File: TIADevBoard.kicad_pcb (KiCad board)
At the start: 2 copper layers, 24.1 x 33 mm, 23 parts, among them J1 Screw_Terminal_01x02, J2 Conn_Coaxial, J3 Conn_Coaxial, J4 Conn_02x03_Counter_Clockwise, J5 Conn_Coaxial, U2 OPA2387, U3 ADP3330-3.3

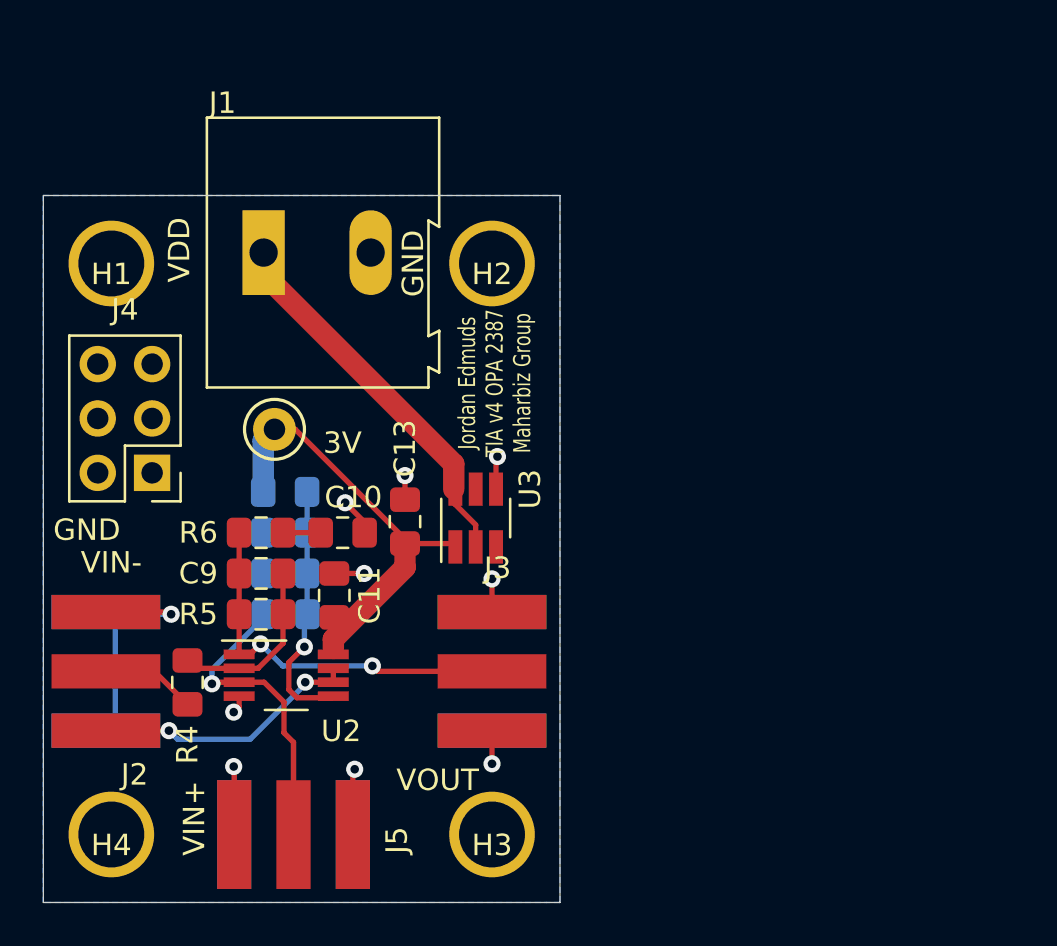
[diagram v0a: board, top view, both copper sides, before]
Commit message: added gerbers for version 5
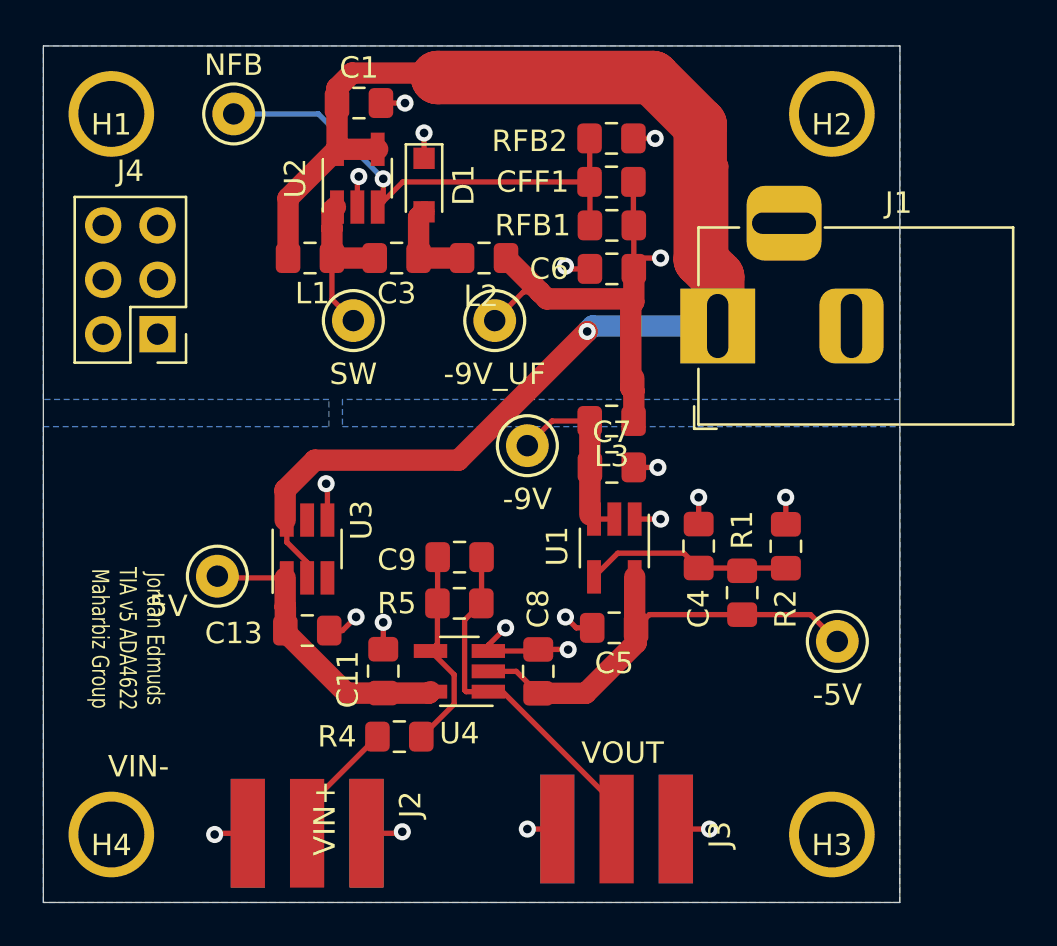
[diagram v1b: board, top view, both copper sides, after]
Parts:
- removed C10: 100pF, Capacitor_SMD:C_0805_2012Metric_Pad1.15x1.40mm_HandSolder
- removed J5: Conn_Coaxial, my_library_foot:CON-SMA-EDGE-S
- removed R3: 0R, Resistor_SMD:R_0805_2012Metric_Pad1.15x1.40mm_HandSolder
- removed R6: 1k, Resistor_SMD:R_0805_2012Metric_Pad1.15x1.40mm_HandSolder
- added C3: 1uF, Capacitor_SMD:C_0805_2012Metric_Pad1.15x1.40mm_HandSolder, F.Cu at (97.1, 82.3)
- added C4: 10nF, Capacitor_SMD:C_0805_2012Metric_Pad1.15x1.40mm_HandSolder, F.Cu at (111.3, 95.7)
- added C5: 10uF, Capacitor_SMD:C_0805_2012Metric_Pad1.15x1.40mm_HandSolder, F.Cu at (107.3, 99.6)
- added C6: 10uF, Capacitor_SMD:C_0805_2012Metric_Pad1.15x1.40mm_HandSolder, F.Cu at (107.2, 82.8)
- added C7: 10uF, Capacitor_SMD:C_0805_2012Metric_Pad1.15x1.40mm_HandSolder, F.Cu at (107.2, 92.1)
- added C8: 100nF, Capacitor_SMD:C_0805_2012Metric_Pad1.15x1.40mm_HandSolder, F.Cu at (103.8, 101.6)
- added CFF1: 100pF, Capacitor_SMD:C_0805_2012Metric_Pad1.15x1.40mm_HandSolder, F.Cu at (107.2, 78.7)
- added D1: D, Diode_SMD:D_SOD-323_HandSoldering, F.Cu at (98.4, 78.9)
- added L1: 22uH, Inductor_SMD:L_0805_2012Metric_Pad1.15x1.40mm_HandSolder, F.Cu at (93.1, 82.3)
- added L2: 22uH, Inductor_SMD:L_0805_2012Metric_Pad1.15x1.40mm_HandSolder, F.Cu at (101.2, 82.3)
- added L3: 22uH, Inductor_SMD:L_0805_2012Metric_Pad1.15x1.40mm_HandSolder, F.Cu at (107.2, 89.9)
- added RFB1: 30k, Resistor_SMD:R_0805_2012Metric_Pad1.15x1.40mm_HandSolder, F.Cu at (107.2, 80.8)
- added RFB2: 4.7k, Resistor_SMD:R_0805_2012Metric_Pad1.15x1.40mm_HandSolder, F.Cu at (107.2, 76.7)
- added TP2: -9V, my_library_foot:TestPoint_Keystone_5000-5004_Miniature, F.Cu at (103.3, 91.1)
- added TP3: -5V, my_library_foot:TestPoint_Keystone_5000-5004_Miniature, F.Cu at (117.7, 100.2)
- added TP4: -9V_UF, my_library_foot:TestPoint_Keystone_5000-5004_Miniature, F.Cu at (101.7, 85.2)
- added TP5: SW, my_library_foot:TestPoint_Keystone_5000-5004_Miniature, F.Cu at (95.1, 85.2)
- added TP6: NFB, my_library_foot:TestPoint_Keystone_5000-5004_Miniature, F.Cu at (89.5, 75.6)
- added U1: TPS723, Package_TO_SOT_SMD:SOT-23-5_HandSoldering, F.Cu at (107.3, 95.8)
- added U4: ADA4622, Package_TO_SOT_SMD:SOT-23-5_HandSoldering, F.Cu at (100.1, 101.6)
- C1: value C -> 10uF; moved to F.Cu
- C11: value 1uF -> 100nF
- J1: value Screw_Terminal_01x02 -> Jack-DC; footprint TerminalBlock:TerminalBlock_Altech_AK300-2_P5.00mm -> Connector_BarrelJack:BarrelJack_Horizontal
- R1: value 10k -> 32k; moved to F.Cu
- R2: value 10k -> 100k; moved to F.Cu
- TP1: value 3V -> 5V
- U2: value OPA2387 -> LM2611; footprint Package_SO:VSSOP-8_3.0x3.0mm_P0.65mm -> Package_TO_SOT_SMD:SOT-23-5_HandSoldering
- U3: value ADP3330-3.3 -> ADP3330-5
- moved U2 23.5 mm to (95.3, 78.6), turned to 90 degrees
- moved R2 23.4 mm to (115.3, 95.8), turned to 90 degrees
- moved R1 21.9 mm to (113.3, 97.9), turned to 90 degrees
- moved J1 21.5 mm to (112.1, 85.5), turned to 180 degrees
- moved C1 20.4 mm to (95.4, 75.1), turned to 0 degrees
- moved H2 17.3 mm to (117.5, 75.6)
- moved H3 15.9 mm to (117.5, 109.2)
- moved R4 10.2 mm to (97.3, 104.6), turned to 180 degrees
- moved J2 9.65 mm to (93.0, 107.4), turned to 90 degrees
- moved J3 9.42 mm to (107.4, 107.2), turned to 90 degrees
- moved C9 9.30 mm to (100.1, 96.3), turned to 180 degrees
- moved R5 9.28 mm to (100.1, 98.4), turned to 180 degrees
- moved U3 8.01 mm to (93.0, 95.9)
- moved TP1 7.36 mm to (88.8, 97.2)
- moved H1 6.98 mm to (83.8, 75.6)
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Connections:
- C1 pad 1: Net-(C1-Pad1) -> VDD
- C11 pad 2: +3V3 -> +5V
- C13 pad 1: +3V3 -> +5V
- J2 pad 2: /VGUARD -> GND
- R1 pad 1: +3V3 -> -5V
- R1 pad 2: Net-(C1-Pad1) -> /VFB
- R2 pad 1: Net-(C1-Pad1) -> /VFB
- TP1 pad 1: +3V3 -> +5V
- U2 pad 1: /VOUT -> Net-(C3-Pad2)
- U2 pad 2: /VOP- -> GND
- U2 pad 3: /VIN+ -> Net-(CFF1-Pad2)
- U2 pad 4: GND -> VDD
- U2 pad 5: Net-(C1-Pad1) -> VDD
- U3 pad 1: +3V3 -> +5V
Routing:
- net VDD: track 17.8 -> 88.9 mm, vias 0 -> 1
- net /VGUARD: track 27.3 -> 0.00 mm, vias 3 -> 0
- net Net-(CFF1-Pad2): track 0.00 -> 24.3 mm, vias 0 -> 1
- net /-9V_UF: track 0.00 -> 22.7 mm, vias 0 -> 1
- net +3V3: track 22.0 -> 0.00 mm
- net -5V: track 0.00 -> 21.6 mm
- net /VIN+: track 15.6 -> 0.00 mm, vias 1 -> 0
- net +5V: track 0.00 -> 13.8 mm
- net GND: track 16.1 -> 28.2 mm, vias 9 -> 19
- net Net-(C1-Pad1): track 11.9 -> 0.00 mm, vias 1 -> 0
- net /VFB: track 0.00 -> 9.71 mm
- net -9V: track 0.00 -> 9.00 mm
- net Net-(C3-Pad2): track 0.00 -> 7.78 mm
- net /DTOP: track 0.00 -> 4.30 mm
- net Net-(C10-Pad1): track 1.76 -> 0.00 mm
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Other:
- board size 24.1 x 33 mm -> 40 x 40 mm
- board text added: "Jordan Edmuds TIA v5 ADA4622 Maharbiz Group"
- board text removed: "GND"
- board text removed: "Jordan Edmuds TIA v4 OPA 2387 Maharbiz Group"
- board text removed: "VDD"
